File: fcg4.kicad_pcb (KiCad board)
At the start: 4 copper layers, 34 x 33.5 mm, 99 parts, among them IC1 MP9943AGQ-Z, IC2 MP9943AGQ-Z, J1 USB4105-GF-A-120, J2 SM08B-SRSS-TB, U1 STM32G473CEUx, U10 MAX40200ANS_T, U11 MAX40200ANS_T, U2 ICM-42688-P, U4 AP2112K-3.3TRG1, U5 AP2112K-1.8TRG1, Y1 ECS-240-6-37B-7KM-TR

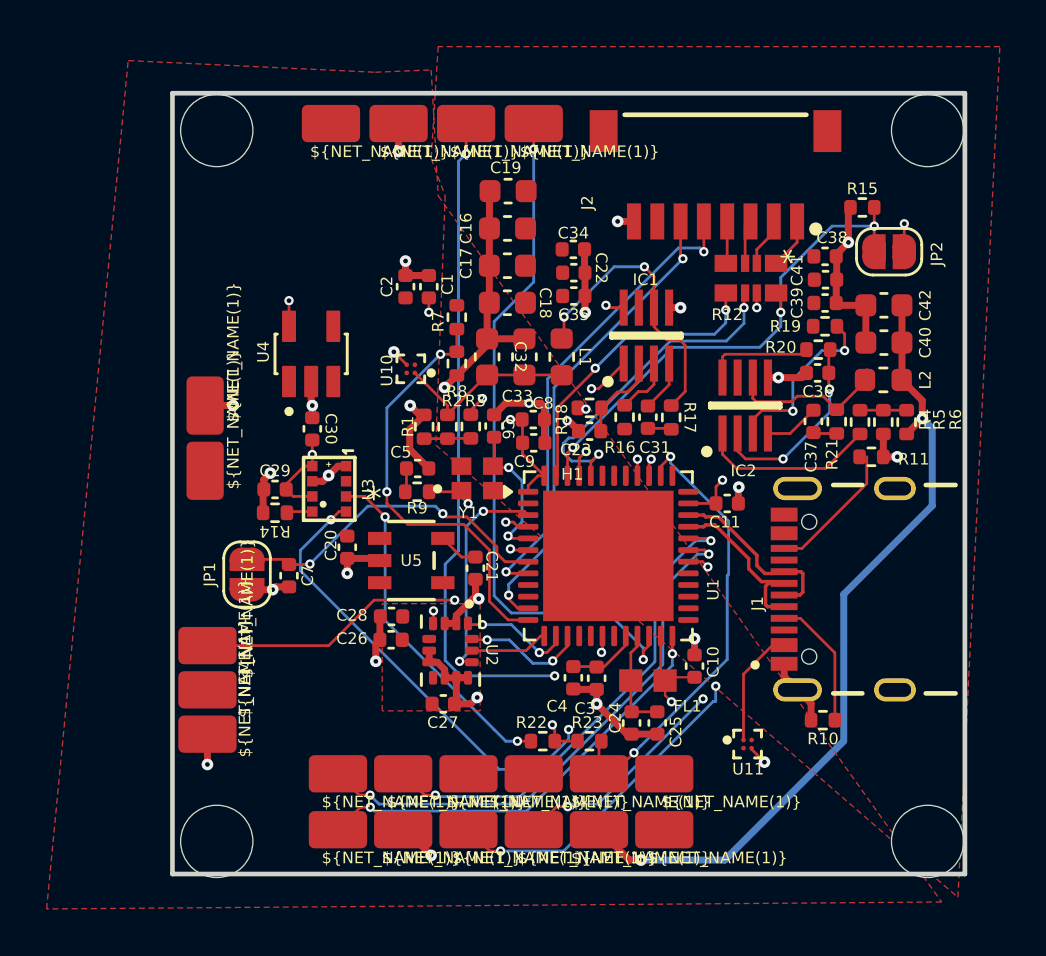
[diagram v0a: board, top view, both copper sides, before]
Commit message: routing
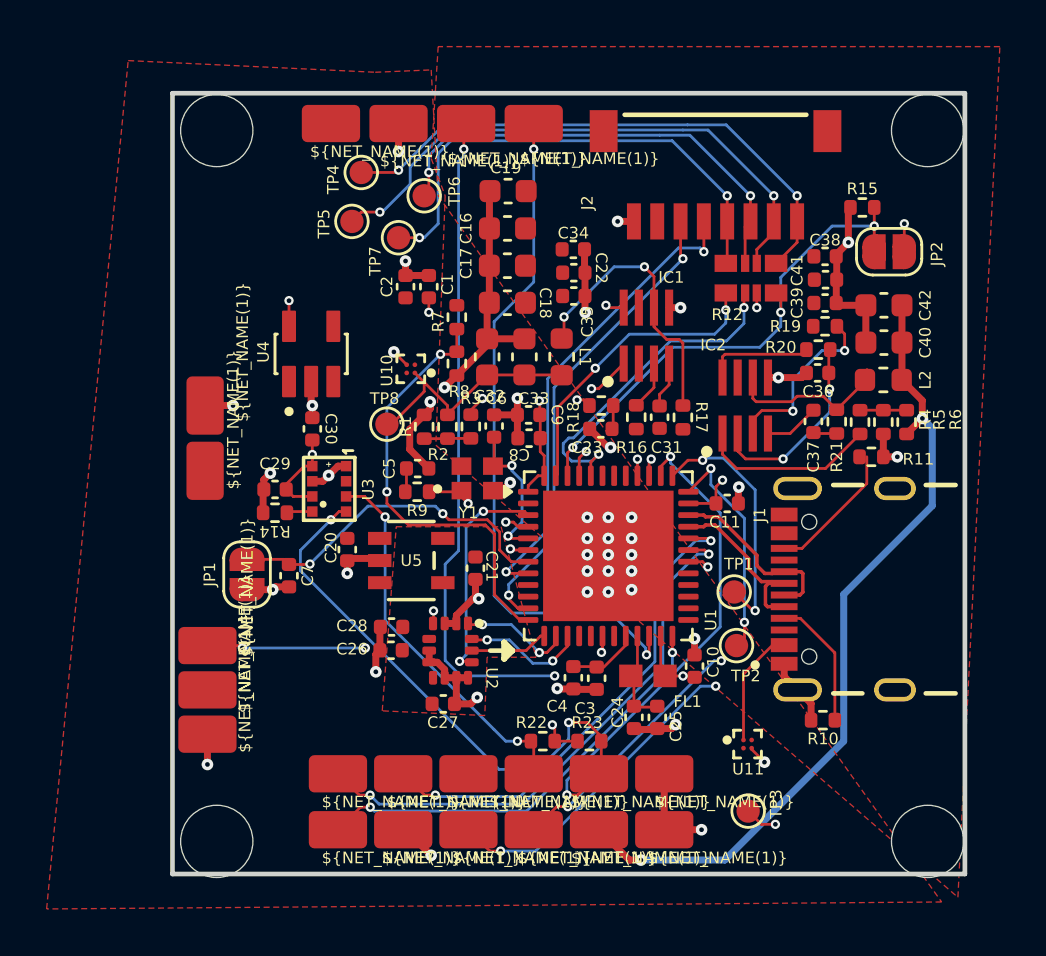
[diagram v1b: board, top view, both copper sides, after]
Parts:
- added TP1: TestPoint, TestPoint:TestPoint_Pad_D1.0mm, F.Cu at (24.2, 21.7)
- added TP2: TestPoint, TestPoint:TestPoint_Pad_D1.0mm, F.Cu at (24.3, 24.0)
- added TP3: TestPoint, TestPoint:TestPoint_Pad_D1.0mm, F.Cu at (24.8, 31.1)
- added TP4: TestPoint, TestPoint:TestPoint_Pad_D1.0mm, F.Cu at (8.20, 3.70)
- added TP5: TestPoint, TestPoint:TestPoint_Pad_D1.0mm, F.Cu at (7.80, 5.80)
- added TP6: TestPoint, TestPoint:TestPoint_Pad_D1.0mm, F.Cu at (10.9, 4.70)
- added TP7: TestPoint, TestPoint:TestPoint_Pad_D1.0mm, F.Cu at (9.80, 6.50)
- added TP8: TestPoint, TestPoint:TestPoint_Pad_D1.0mm, F.Cu at (9.30, 14.5)
- moved C9 1.22 mm to (15.4, 14.1), turned to 180 degrees
- moved C8 0.82 mm to (15.4, 15.1), turned to 180 degrees
- moved R18 0.51 mm to (18.5, 13.7)
- moved C31 0.50 mm to (21.0, 14.2)
- moved R16 0.50 mm to (20.0, 14.2)
- moved R17 0.50 mm to (22.0, 14.2)
- moved C23 0.49 mm to (18.5, 14.7)
- moved C26 0.45 mm to (9.48, 24.2)
- moved C28 0.45 mm to (9.50, 23.2)
- moved C24 0.26 mm to (19.9, 27.1)
- moved C25 0.24 mm to (20.9, 27.1)
- moved FL1 0.20 mm to (20.5, 25.3)
- moved C20 0.10 mm to (7.60, 19.9)
- turned H1 to 90 degrees
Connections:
- net BEEPER renamed BZ
- C21 pad 1: /Power/VOUT -> VCC_ICM
- U1 pad 36: PINIO1 -> SWDIO-JTMS
- U1 pad 37: unconnected-(U1-PA14-Pad37) -> SWCLK-JTCK
- U5 pad 5: /Power/VOUT -> VCC_ICM
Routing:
- net /Connectors/MOTOR_2: track 2.10 -> 24.8 mm, vias 0 -> 2
- net /Connectors/MOTOR_1: track 2.17 -> 24.1 mm, vias 0 -> 2
- net /Connectors/MOTOR_4: track 1.82 -> 21.5 mm, vias 0 -> 2
- net /Connectors/MOTOR_3: track 1.90 -> 20.0 mm, vias 0 -> 2
- net SWCLK-JTCK: track 0.00 -> 10.8 mm, vias 0 -> 2
- net SWDIO-JTMS: track 0.00 -> 9.74 mm, vias 0 -> 2
- net GND: track 70.3 -> 73.3 mm, vias 28 -> 46
- net 5V5_BEC: track 8.00 -> 10.6 mm
- net /Power/BIAS_SUPPLY_5V5: track 3.83 -> 1.83 mm
- net I2C1_SCL: track 43.5 -> 45.2 mm
- net /Power/VOUT: track 1.73 -> 0.00 mm
- net I2C1_SDA: track 26.0 -> 27.5 mm
- net /Power/RC_BST_5V5: track 0.96 -> 0.00 mm
- net TX4: track 23.1 -> 22.6 mm
- net TX3: track 30.1 -> 29.6 mm
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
